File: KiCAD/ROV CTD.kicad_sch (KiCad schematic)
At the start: 43 parts, among them J1 Conn_Coaxial, J10 1Wire1, J11 1Wire2, J12 1Wire3, J13 Interface, J14 Interface, J15 Conn_01x07_Pin, J6 Main In, M1 EZO-EC, M2 MS5803-14BA, U2 ATtiny1614-Arduino, U3 AP63205WU, U6 MAX3072E

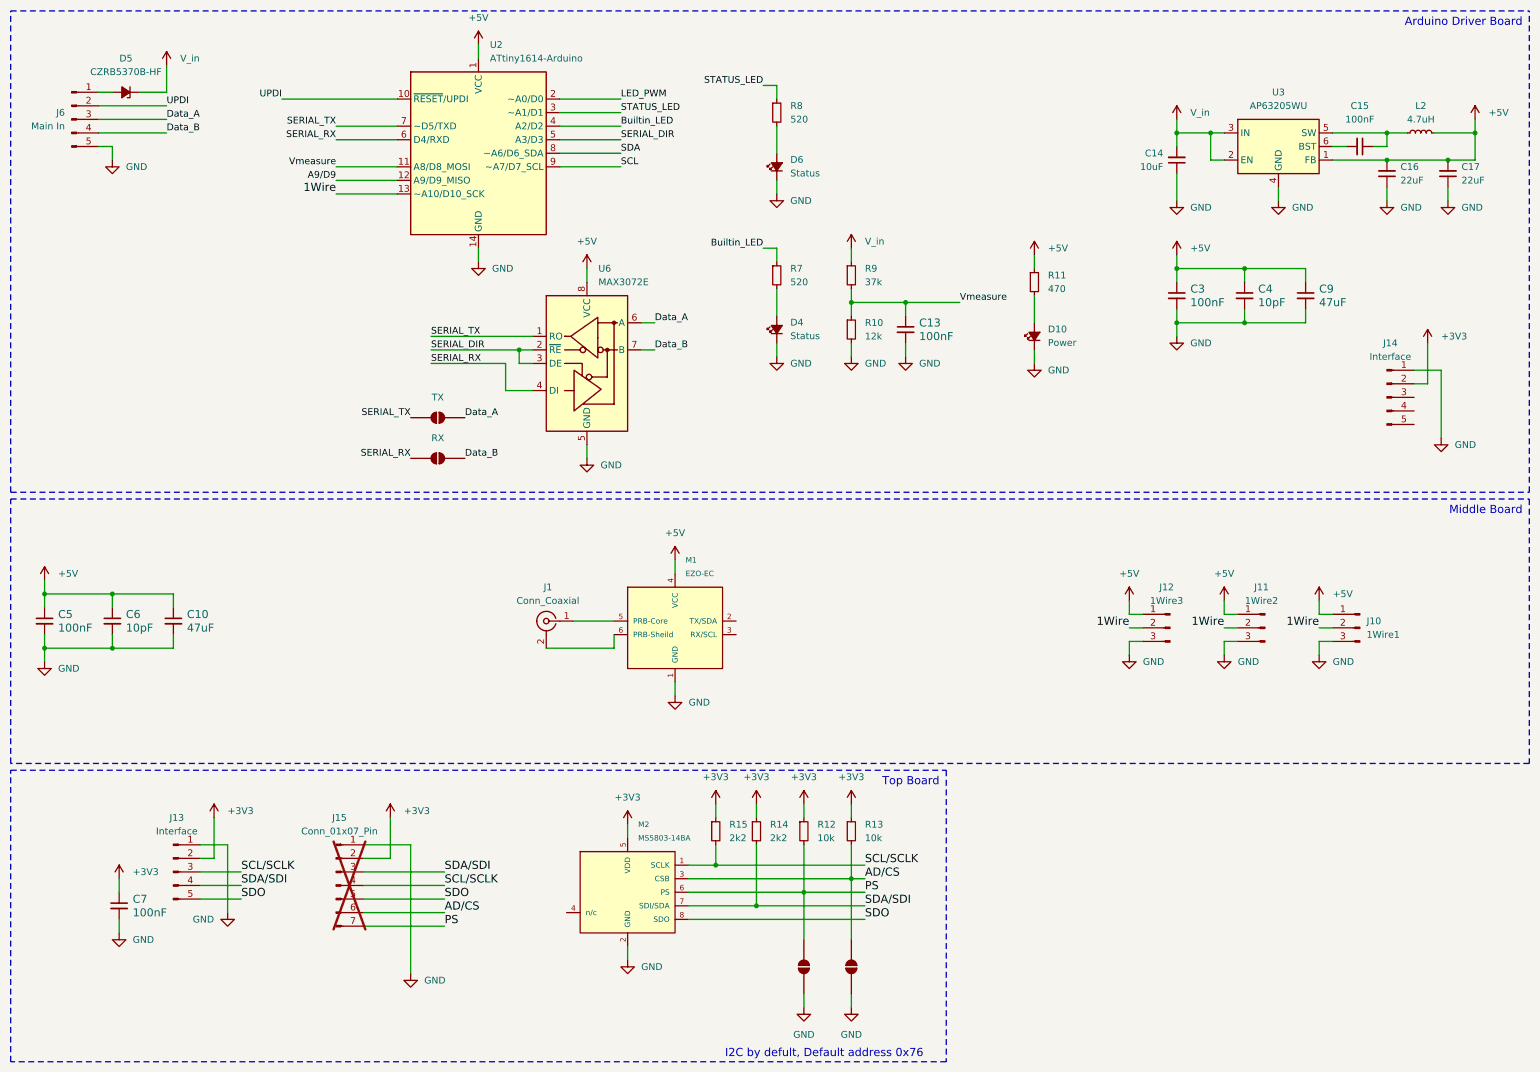
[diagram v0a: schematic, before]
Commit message: .
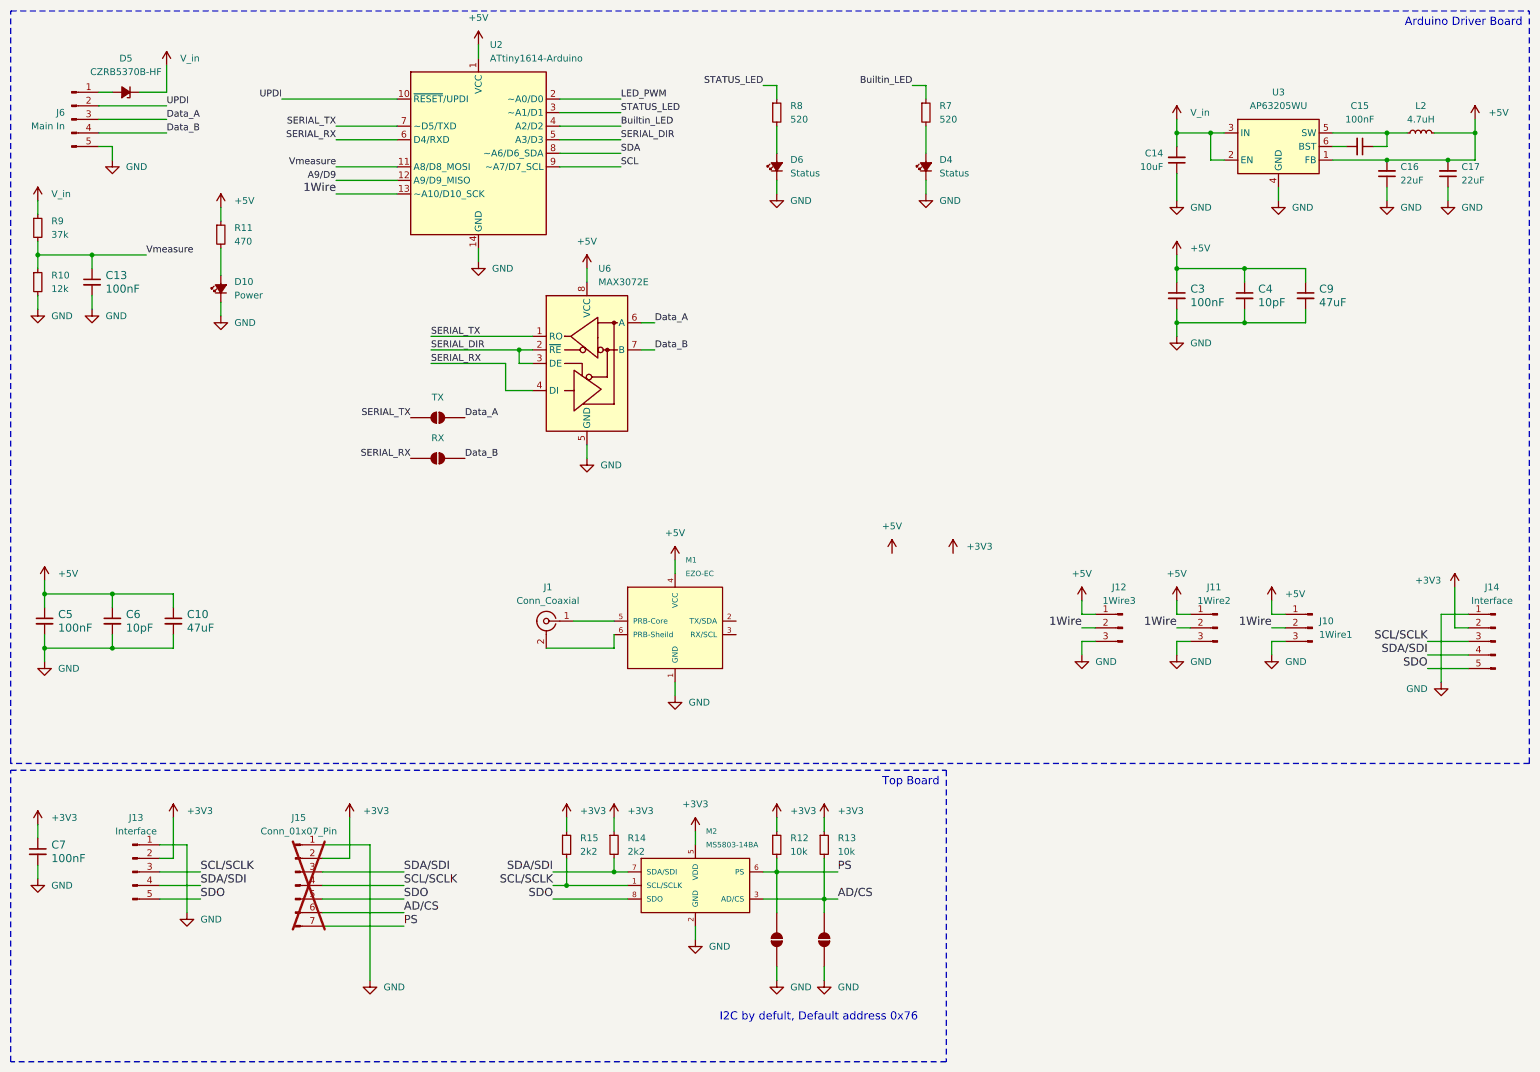
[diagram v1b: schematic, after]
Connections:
- net SCL/SCLK: now also J14.3 (Pin_3)
- net SDA/SDI: now also J14.4 (Pin_4)
- net SDO: now also J14.5 (Pin_5)
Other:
- note removed: "Middle Board"
- moved on the sheet: C13, C7, D10, D4, J10, J11, J12, J13, J14, J15, R10, R11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
